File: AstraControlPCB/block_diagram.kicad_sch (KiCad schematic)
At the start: 0 parts

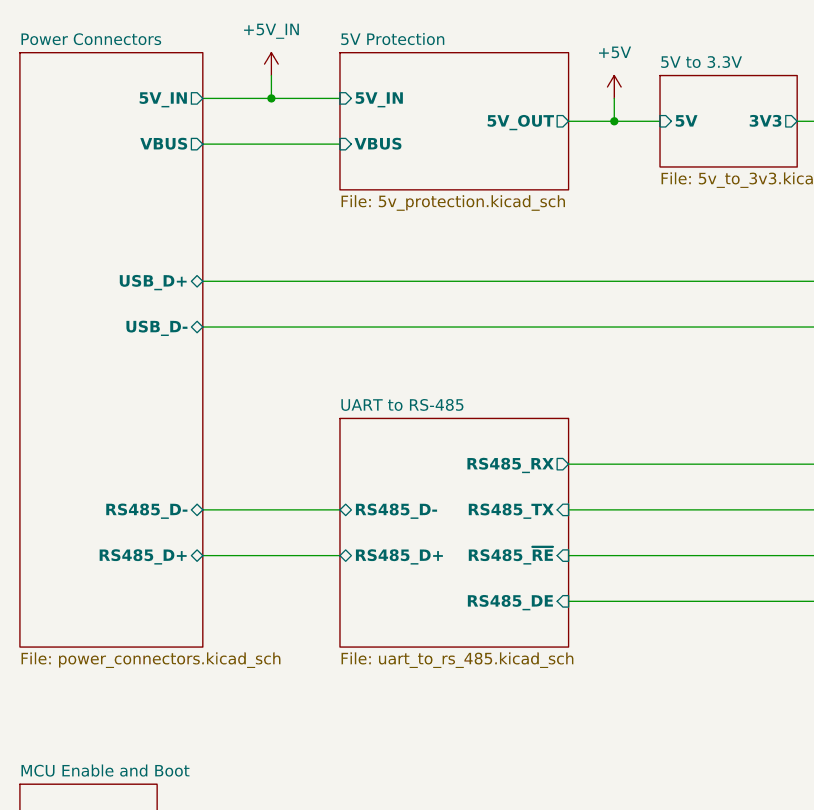
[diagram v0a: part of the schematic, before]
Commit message: Another redesign
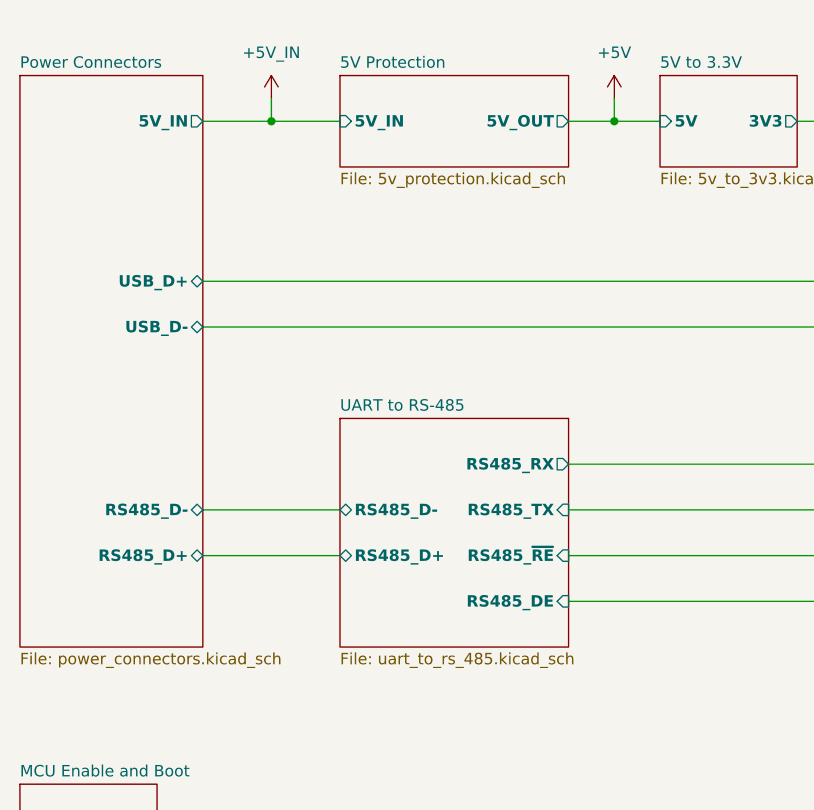
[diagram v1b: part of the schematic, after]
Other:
- sheet 5V Protection ports: added none; removed VBUS
- sheet Power Connectors ports: added none; removed VBUS
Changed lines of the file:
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@@
 	)
 	(junction
-		(at 45.72 27.94)
+		(at 45.72 30.48)
 		(diameter 0)
 		(color 0 0 0 0)
@@
 	(wire
 		(pts
-			(xy 38.1 27.94) (xy 45.72 27.94)
+			(xy 38.1 30.48) (xy 45.72 30.48)
 		)
 		(stroke
@@
 		)
 	)
-	(wire
-		(pts
-			(xy 38.1 33.02) (xy 53.34 33.02)
-		)
-		(stroke
-			(width 0)
-			(type default)
-		)
-	)
 	(polyline
 		(pts
@@
 	(wire
 		(pts
-			(xy 45.72 25.4) (xy 45.72 27.94)
+			(xy 45.72 27.94) (xy 45.72 30.48)
 		)
 		(stroke
@@
 	(wire
 		(pts
-			(xy 45.72 27.94) (xy 53.34 27.94)
+			(xy 45.72 30.48) (xy 53.34 30.48)
 		)
 		(stroke
@@
 	(symbol
 		(lib_id "LiveAstra:+5V_IN")
-		(at 45.72 25.4 0)
+		(at 45.72 27.94 0)
 		(unit 1)
 		(exclude_from_sim no)
@@
 		(fields_autoplaced yes)
 		(property "Reference" "#PWR01"
-			(at 45.72 29.21 0)
+			(at 45.72 31.75 0)
 			(effects
 				(font
@@
 		)
 		(property "Value" "+5V_IN"
-			(at 45.72 20.32 0)
+			(at 45.72 22.86 0)
 			(effects
 				(font
@@
 		)
 		(property "Footprint" ""
-			(at 45.72 25.4 0)
+			(at 45.72 27.94 0)
 			(effects
 				(font
@@
 		)
 		(property "Datasheet" ""
-			(at 45.72 25.4 0)
+			(at 45.72 27.94 0)
 			(effects
 				(font
@@
 		)
 		(property "Description" "Power symbol creates a global label with name \"+5V_IN\""
-			(at 45.72 25.4 0)
+			(at 45.72 27.94 0)
 			(effects
 				(font
@@
 	)
 	(sheet
-		(at 17.78 22.86)
-		(size 20.32 66.04)
+		(at 17.78 25.4)
+		(size 20.32 63.5)
 		(fields_autoplaced yes)
 		(stroke
@@
 		)
 		(property "Sheetname" "Power Connectors"
-			(at 17.78 22.1484 0)
+			(at 17.78 24.6884 0)
 			(effects
 				(font
@@
 		)
 		(pin "5V_IN" output
-			(at 38.1 27.94 0)
-			(effects
-				(font
-					(size 1.27 1.27)
-					(thickness 0.254)
-					(bold yes)
-				)
-				(justify right)
-			)
-		)
-		(pin "VBUS" output
-			(at 38.1 33.02 0)
+			(at 38.1 30.48 0)
 			(effects
 				(font
@@
 	)
 	(sheet
-		(at 53.34 22.86)
-		(size 25.4 15.24)
+		(at 53.34 25.4)
+		(size 25.4 10.16)
 		(fields_autoplaced yes)
 		(stroke
@@
 		)
 		(property "Sheetname" "5V Protection"
-			(at 53.34 22.1484 0)
+			(at 53.34 24.6884 0)
 			(effects
 				(font
@@
 		)
 		(property "Sheetfile" "5v_protection.kicad_sch"
-			(at 53.34 38.6846 0)
+			(at 53.34 36.1446 0)
 			(effects
 				(font
@@
 		)
 		(pin "5V_IN" input
-			(at 53.34 27.94 180)
+			(at 53.34 30.48 180)
 			(effects
 				(font
@@
 			)
 		)
-		(pin "VBUS" input
-			(at 53.34 33.02 180)
-			(effects
-				(font
-					(size 1.27 1.27)
-					(thickness 0.254)
-					(bold yes)
-				)
-				(justify left)
-			)
-		)
